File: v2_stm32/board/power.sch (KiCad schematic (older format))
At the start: 24 parts, among them U2 MP2451DT-LF-Z, U3 LM317_TO-252, U4 AMS1117-3.3

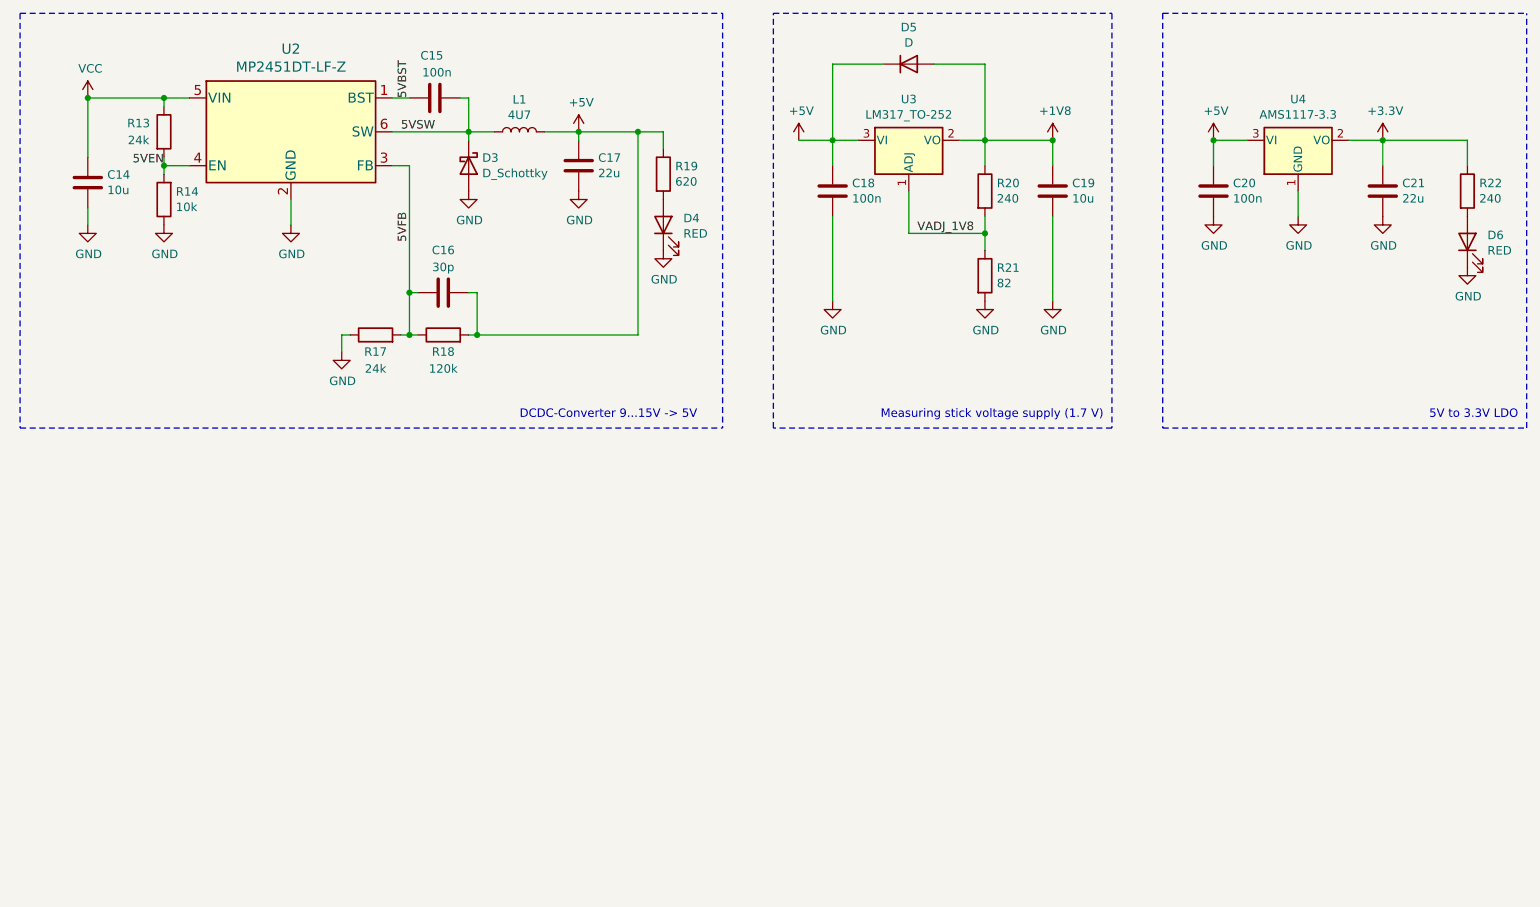
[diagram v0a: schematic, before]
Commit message: More PCB design
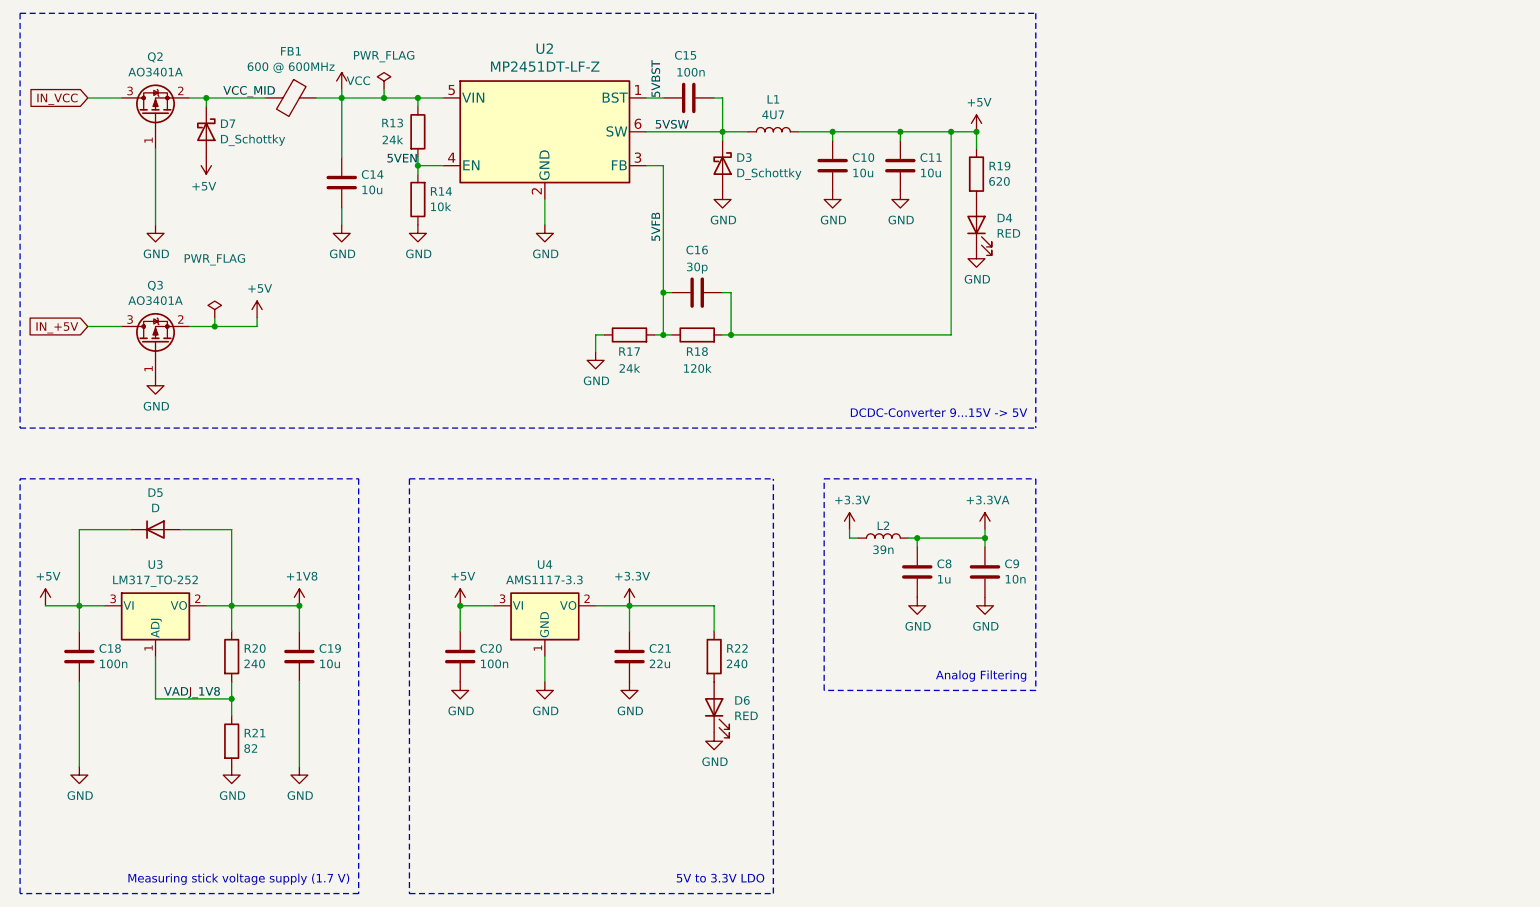
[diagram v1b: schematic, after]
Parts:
- removed C17: 22u, Capacitor_SMD:C_0805_2012Metric, symbol Device:C
- added C10, C11: 10u, Capacitor_SMD:C_0805_2012Metric, symbol Device:C
- added C8: 1u, Inductor_SMD:L_0402_1005Metric, symbol Device:C
- added C9: 10n, Inductor_SMD:L_0402_1005Metric, symbol Device:C
- added D7: D_Schottky, Diode_SMD:D_SOD-123, symbol Device:D_Schottky
- added FB1: 600 @ 600MHz, Inductor_SMD:L_0805_2012Metric, symbol Device:Ferrite_Bead
- added L2: 39n, Inductor_SMD:L_0402_1005Metric, symbol Device:L
- added Q2, Q3: AO3401A, Package_TO_SOT_SMD:SOT-23, symbol Transistor_FET:AO3401A
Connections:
- net +3V3: now also L2.1
- net +5V: now also C10.1, C11.1, D7.2 (A), Q3.2 (S)
- net GND: now also C10.2, C11.2, C8.2, C9.2, Q2.1 (G), Q3.1 (G)
- net VCC: now also FB1.1
- new net +3.3VA: C8.1, C9.1, L2.2
- new net IN_+5V: Q3.3 (D)
- new net IN_VCC: Q2.3 (D)
- new net VCC_MID: D7.1 (K), FB1.2, Q2.2 (S)
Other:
- note added: "Analog Filtering"
- moved on the sheet: C14, C15, C16, C18, C19, C20, C21, D3, D4, D5, D6, L1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
